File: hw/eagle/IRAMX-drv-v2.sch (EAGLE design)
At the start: 64 parts, among them IC1 IRAMTOP, IC3 LM393N, IC4 4049N, IC5 4013N, IC6 7805, IC7 7815, Q1 IRF740

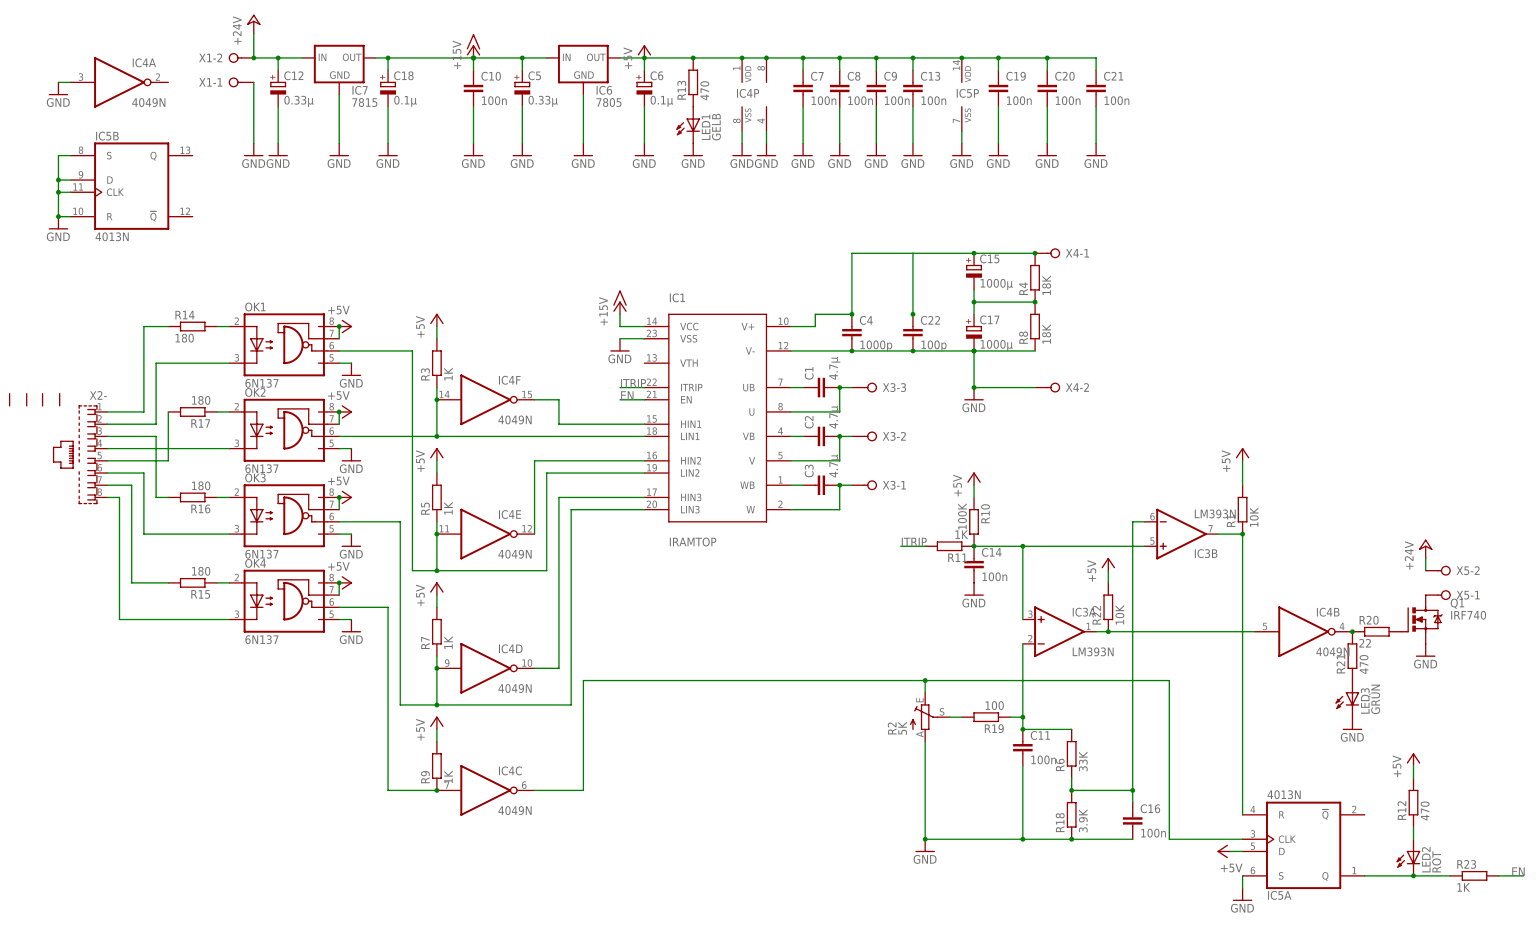
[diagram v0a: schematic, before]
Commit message: r net
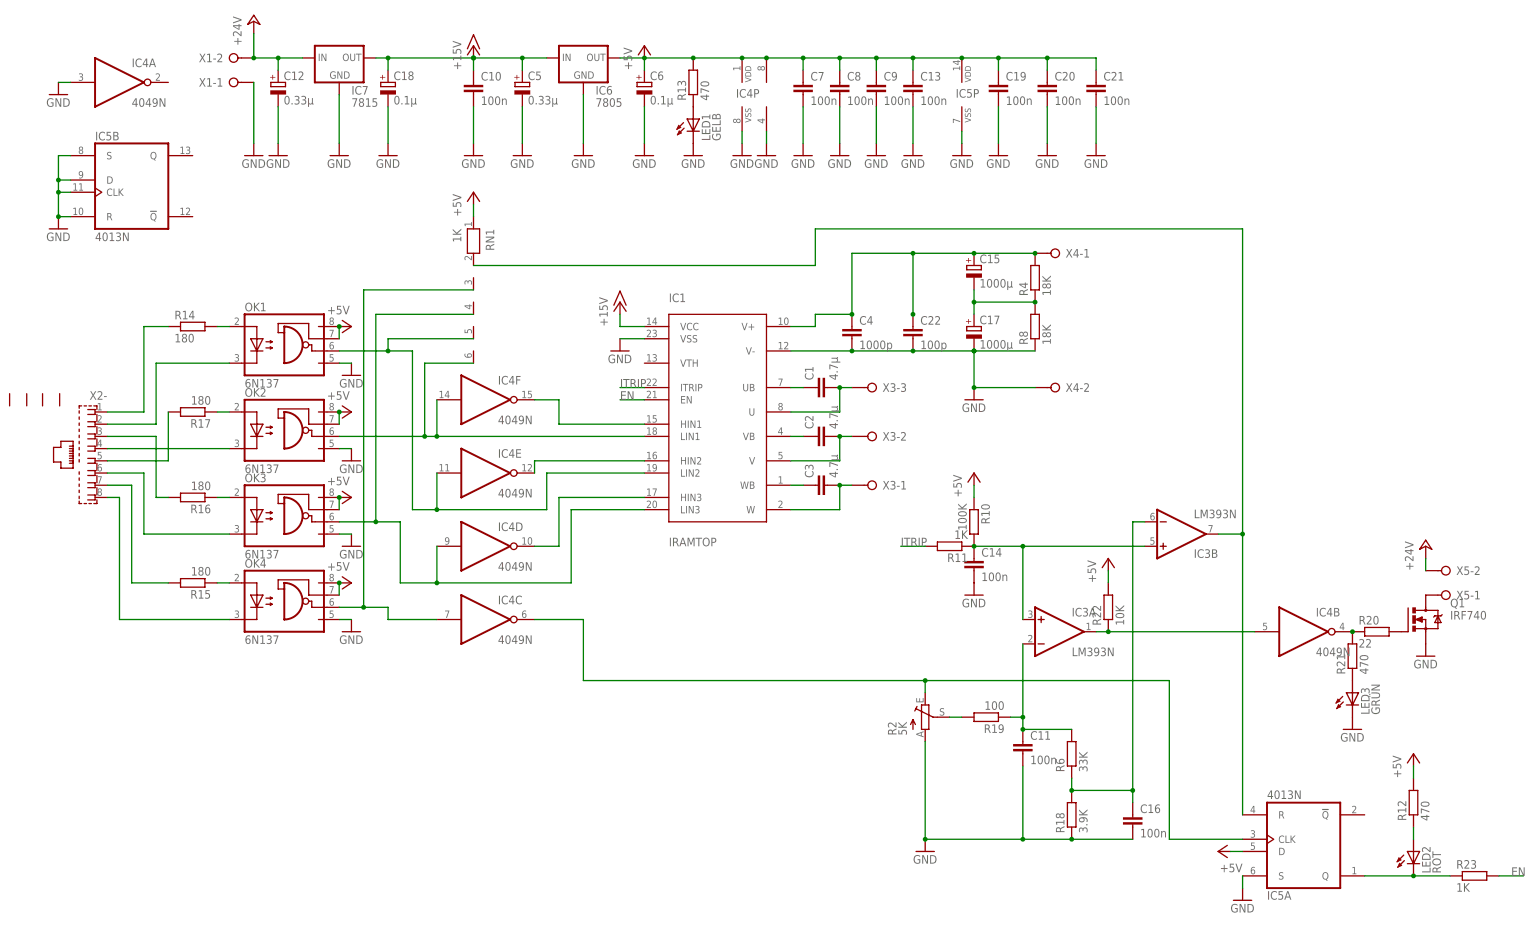
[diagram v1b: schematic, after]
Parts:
- removed R1: 10K, rcl:R-EU_0204/7
- removed R3, R5, R7, R9: 1K, rcl:R-EU_0204/7
- added RN1: 1K, resistor-net:RN05
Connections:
- net +5V: now also RN1.1; no longer R1.2, R3.2, R5.2, R7.2, R9.2
- net N$24: now also RN1.6; no longer R3.1
- net N$29: now also RN1.3; no longer R9.1
- net N$35: now also RN1.5; no longer R5.1
- net N$38: now also RN1.4; no longer R7.1
- net N$42: now also RN1.2; no longer R1.1
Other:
- moved on the sheet: IC4C, IC4D, IC4E
